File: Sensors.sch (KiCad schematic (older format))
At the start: 35 parts, among them CN3 CONN_HEADER_SMD_4POS_2MM, CN4 CONN_HEADER_SMD_4POS_2MM, U1 LPS25HB, U10 MPXV4006GP, U11 MPXV4006DP, U12 TLV2333IDR, U17 MPXV4006GP

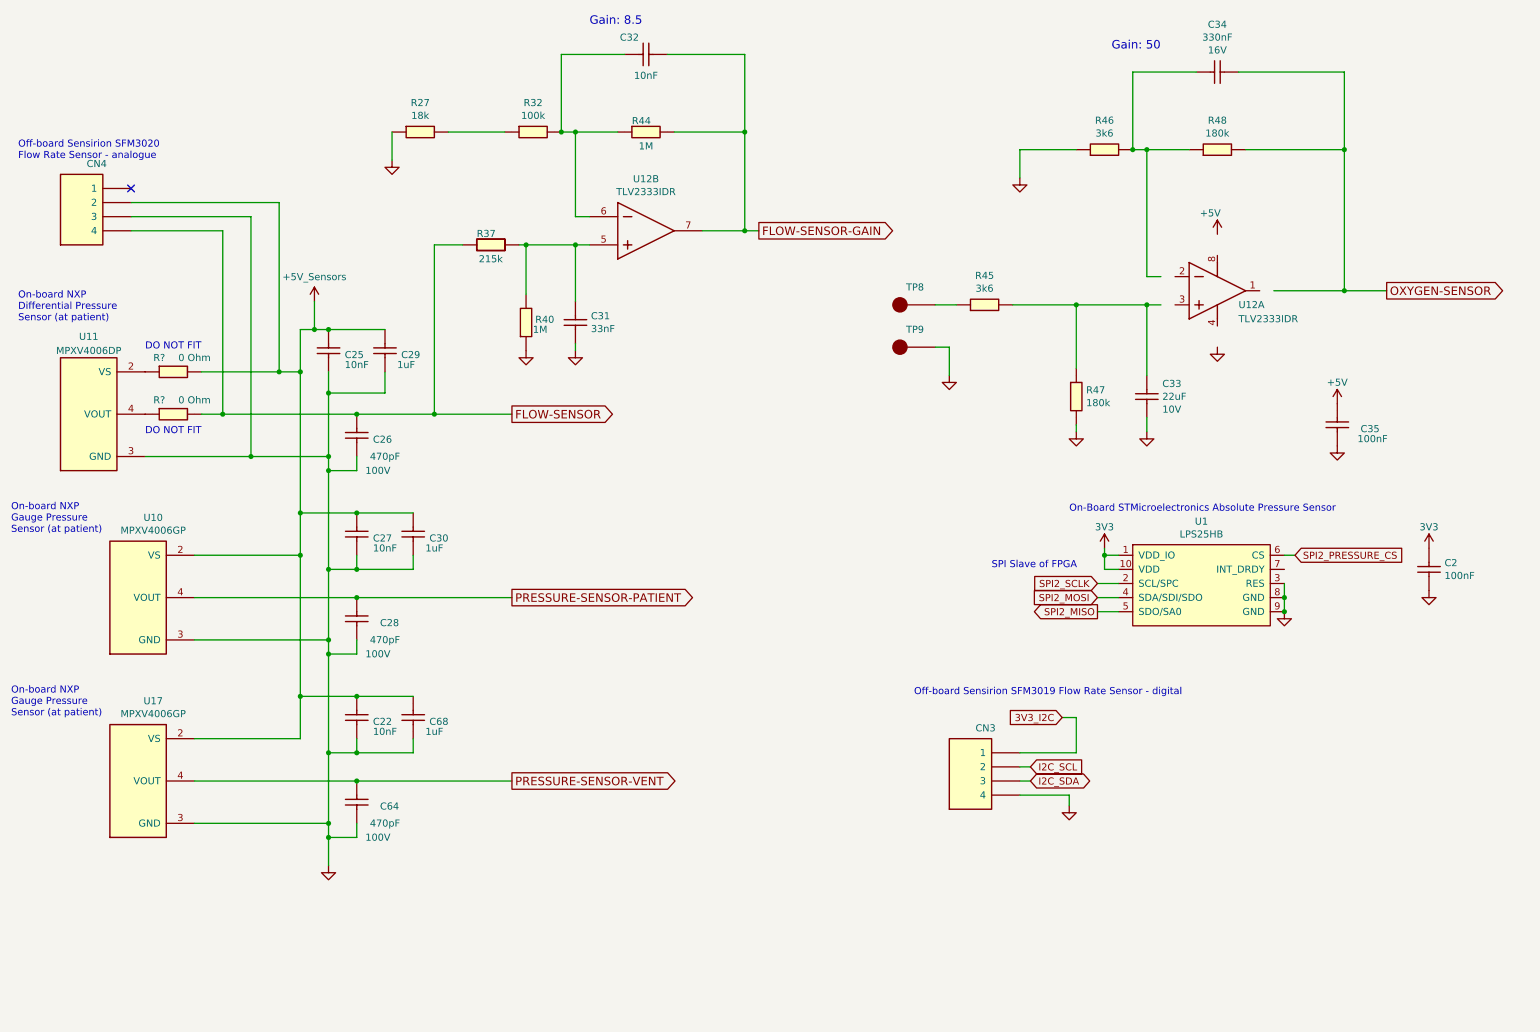
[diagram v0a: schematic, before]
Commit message: Rick's changes - April 19
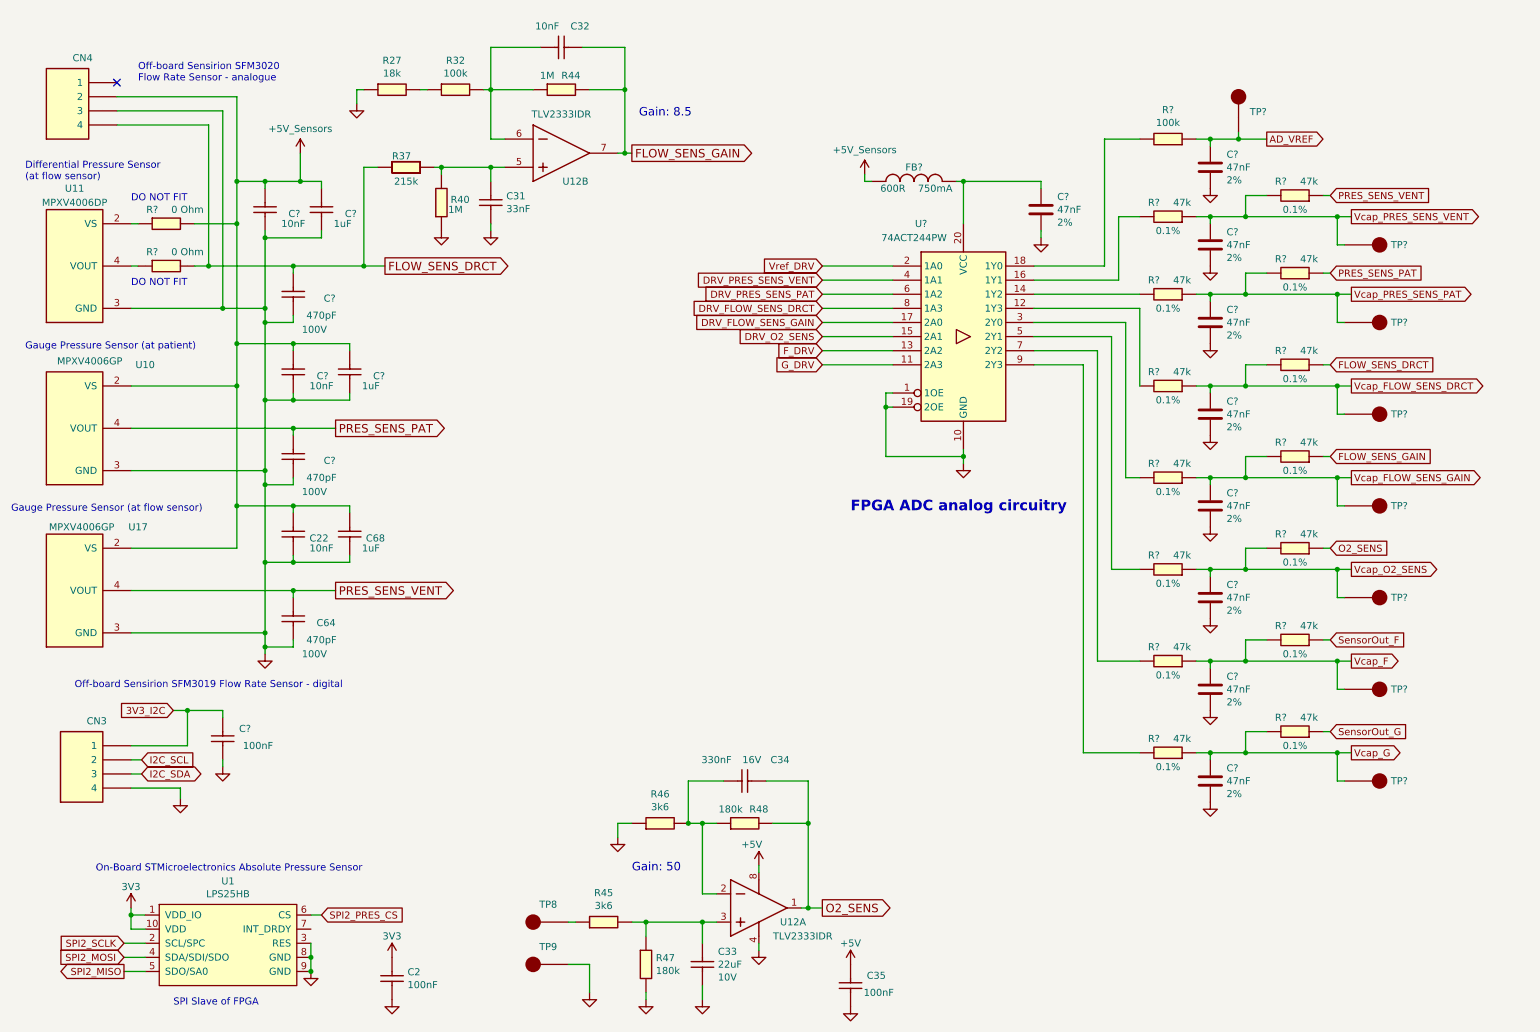
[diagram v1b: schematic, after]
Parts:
- removed C25, C27: 10nF_0603_Ceramic_Capacitor,_10%,_50V,_X7R-, Capacitor_SMD:C_0603_1608Metric, symbol OpenVent:10nF_0603_Ceramic_Capacitor,_10%,_50V,_X7R-
- removed C26, C28: 470pF_0603_Ceramic_Capacitor,_5%,_100V,_C0G, Capacitor_SMD:C_0603_1608Metric, symbol OpenVent:470pF_0603_Ceramic_Capacitor,_5%,_100V,_C0G
- removed C29, C30: 1uF_0603_Ceramic_Capacitor,_10%,_50V,_X5R, Capacitor_SMD:C_0603_1608Metric, symbol OpenVent:1uF_0603_Ceramic_Capacitor,_10%,_50V,_X5R
- added C? (x2): 470pF_0603_Ceramic_Capacitor,_5%,_100V,_C0G, Capacitor_SMD:C_0603_1608Metric, symbol OpenVent:470pF_0603_Ceramic_Capacitor,_5%,_100V,_C0G
- added C? (x2): 1uF_0603_Ceramic_Capacitor,_10%,_50V,_X5R, Capacitor_SMD:C_0603_1608Metric, symbol OpenVent:1uF_0603_Ceramic_Capacitor,_10%,_50V,_X5R
- added C? (x2): 10nF_0603_Ceramic_Capacitor,_10%,_50V,_X7R-, Capacitor_SMD:C_0603_1608Metric, symbol OpenVent:10nF_0603_Ceramic_Capacitor,_10%,_50V,_X7R-
- added C? (x9): C_1206_47nF_16V_2%_PPS_film, Capacitor_SMD:C_1206_3216Metric, symbol OpenVent:C_1206_47nF_16V_2%_PPS_film
- added C?: 100nF_0603_Ceramic_Capacitor,_10%,_X7R,_25V, Capacitor_SMD:C_0603_1608Metric, symbol OpenVent:100nF_0603_Ceramic_Capacitor,_10%,_X7R,_25V
- added FB?: Chip_Ferrite,_600R,_0603,_750mA, symbol OpenVent:Chip_Ferrite,_600R,_0603,_750mA
- added R?: 100K_0603_Chip_Resistor,_1%,_0.1W, symbol OpenVent:100K_0603_Chip_Resistor,_1%,_0.1W
- added R? (x14): R_0603_47K_0.1%_0.1W_Film, Resistor_SMD:R_0603_1608Metric_Pad0.98x0.95mm_HandSolder, symbol OpenVent:R_0603_47K_0.1%_0.1W_Film
- added TP? (x8): Test_Point_PTH, symbol OpenVent:Test_Point_PTH
- added U?: 74ACT244PW, symbol OpenVent:74ACT244PW
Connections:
- net OXYGEN-SENSOR is gone; now on net O2_SENS: C34.2, R48.2
- net +5V: now also U12.8 (V+), C?.2, C?.2, C?.2, C?.2, FB?.1
- net 3V3_I2C: now also C?.2
- net GND: now also U12.4 (V-), C?.1, C?.1, C?.1, C?.1, C?.1, C?.1, C?.1, C?.2, C?.2, C?.2, C?.2, C?.2, C?.2, C?.2, C?.2, C?.2, U?.1 (1OE), U?.10 (GND), U?.19 (2OE)
- net O2_SENS: now reaches U12.1 (OUTA)
- net O2_SENS: now also R?.1
- net at U12.2 (INA-): now also C34.1, R46.2, R48.1
- net at U12.3 (INA+): now also C33.1, R45.2, R47.1
- net FLOW-SENSOR renamed FLOW_SENS_DRCT
- net FLOW_SENS_DRCT: now also C?.2, R?.1
- net FLOW-SENSOR-GAIN renamed FLOW_SENS_GAIN
- net FLOW_SENS_GAIN: now also R?.1
- net PRESSURE-SENSOR-PATIENT renamed PRES_SENS_PAT
- net PRES_SENS_PAT: now also C?.2, R?.1
- net PRESSURE-SENSOR-VENT renamed PRES_SENS_VENT
- net PRES_SENS_VENT: now also R?.1
- net SPI2_PRESSURE_CS renamed SPI2_PRES_CS
- new net: R?.2, U?.18 (1Y0)
- new net: C?.1, FB?.2, U?.20 (VCC)
- new net: R?.2, U?.9 (2Y3)
- new net: R?.2, U?.12 (1Y3)
- new net: R?.2, U?.14 (1Y2)
- new net: R?.2, U?.16 (1Y1)
- new net: R?.2, U?.3 (2Y0)
- new net: R?.2, U?.5 (2Y1)
- new net: R?.2, U?.7 (2Y2)
- new net AD_VREF: C?.1, R?.1, TP?.1
- new net DRV_FLOW_SENS_DRCT: U?.8 (1A3)
- new net DRV_FLOW_SENS_GAIN: U?.17 (2A0)
- new net DRV_O2_SENS: U?.15 (2A1)
- new net DRV_PRES_SENS_PAT: U?.6 (1A2)
- new net DRV_PRES_SENS_VENT: U?.4 (1A1)
- new net F_DRV: U?.13 (2A2)
- new net G_DRV: U?.11 (2A3)
- new net SensorOut_F: R?.1
- new net SensorOut_G: R?.1
- new net Vcap_F: C?.1, R?.1, R?.2, TP?.1
- new net Vcap_FLOW_SENS_DRCT: C?.1, R?.1, R?.2, TP?.1
- new net Vcap_FLOW_SENS_GAIN: C?.1, R?.1, R?.2, TP?.1
- new net Vcap_G: C?.1, R?.1, R?.2, TP?.1
- new net Vcap_O2_SENS: C?.1, R?.1, R?.2, TP?.1
- new net Vcap_PRES_SENS_PAT: C?.1, R?.1, R?.2, TP?.1
- new net Vcap_PRES_SENS_VENT: C?.1, R?.1, R?.2, TP?.1
- new net Vref_DRV: U?.2 (1A0)
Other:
- note added: "Differential Pressure Sensor\n(at flow sensor)"
- note added: "FPGA ADC analog circuitry"
- note added: "Gauge Pressure Sensor (at flow sensor)"
- note added: "Gauge Pressure Sensor (at patient)"
- note removed: "On-board NXP\nDifferential Pressure\nSensor (at patient)"
- note removed: "On-board NXP\nGauge Pressure\nSensor (at patient)"
- moved on the sheet: C2, C22, C31, C32, C33, C34, C35, C64, C68, CN3, CN4, R27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
